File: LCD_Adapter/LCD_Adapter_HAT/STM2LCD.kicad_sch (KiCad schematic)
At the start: 45 parts, among them J1 2-84953-0, J2 FH12-30S-0.5SH_55_, J3 RPi_GPIO, J4 Conn_02x20_Odd_Even, Q1 2N7002, Q2 2N7002, U4 PCA9306DCURG4

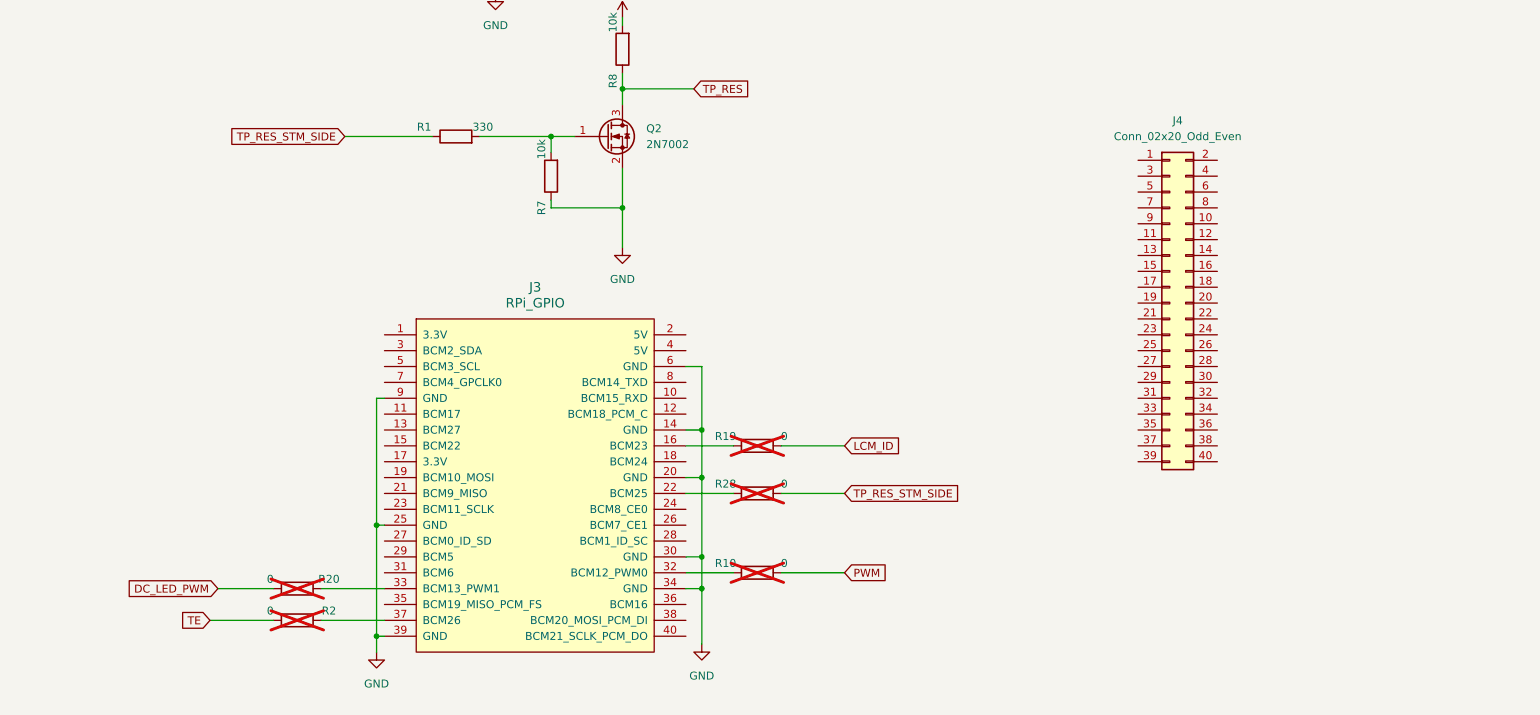
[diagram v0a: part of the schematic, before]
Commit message: PCB_UPDATE
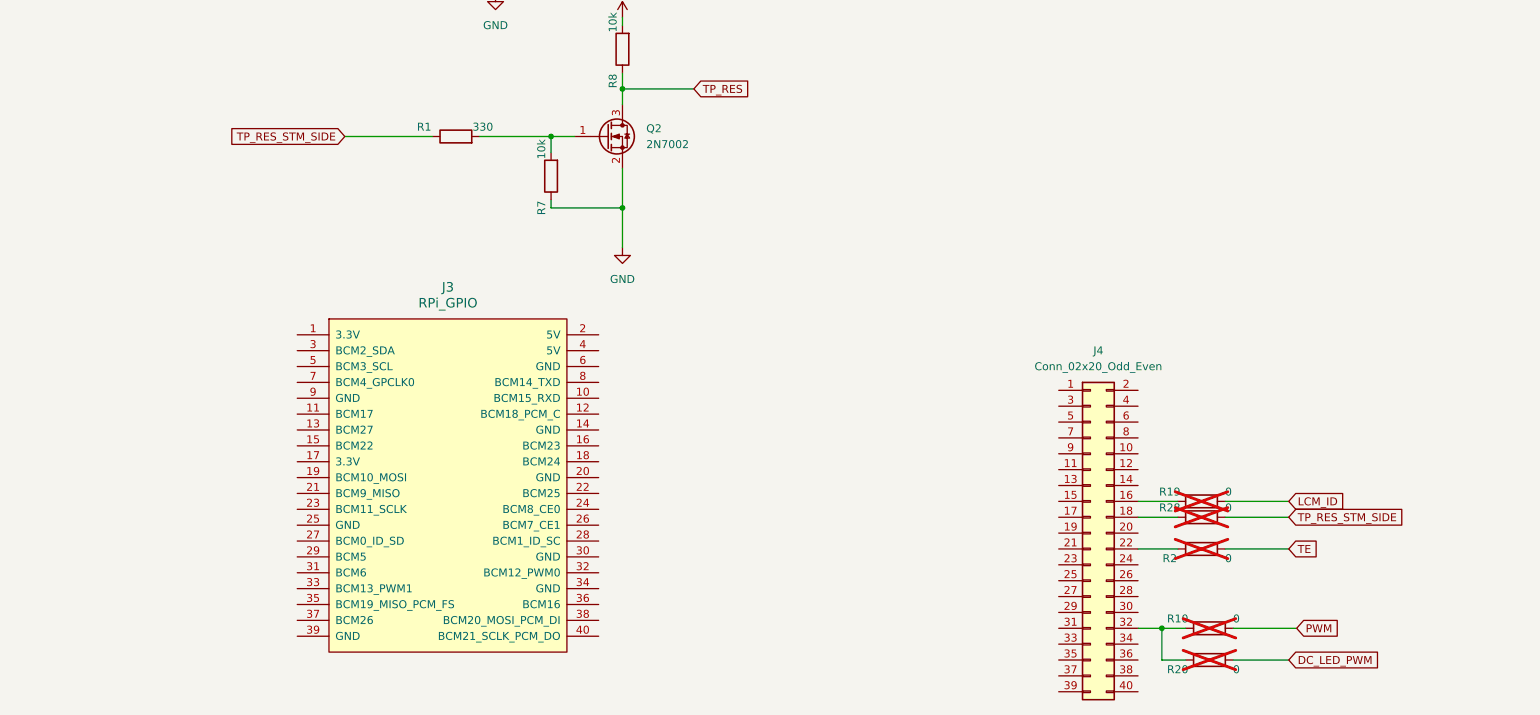
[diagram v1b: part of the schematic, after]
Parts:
- J3, TP1, TP15, TP16, TP2, TP3, TP4, TP5, TP6: now left out of the parts list
- J4: LCSC# (none) -> C2685092
- R10, R19, R2, R20, R24, R25, R26, R27, R28, R4, R5: LCSC# (none) -> C21189
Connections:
- net GND: no longer J3.14 (GND), J3.20 (GND), J3.25 (GND), J3.30 (GND), J3.34 (GND), J3.39 (GND), J3.6 (GND), J3.9 (GND)
- net at R19.1: now also J4.16 (Pin_16); no longer J3.16 (BCM23)
- net at R2.1: now also J4.22 (Pin_22); no longer J3.37 (BCM26)
- net at J3.22 (BCM25): no longer R28.1
- net at J3.32 (BCM12_PWM0): no longer R10.1
- net at J3.33 (BCM13_PWM1): no longer R20.1
- net at J4.18 (Pin_18): now also R28.1
- net at J4.32 (Pin_32): now also R10.1, R20.1
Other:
- moved on the sheet: J3, J4, R10, R19, R2, R20, R28
